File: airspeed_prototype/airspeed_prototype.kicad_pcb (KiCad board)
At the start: 2 copper layers, 2 parts, among them U1 BME280, U2 ADXL343

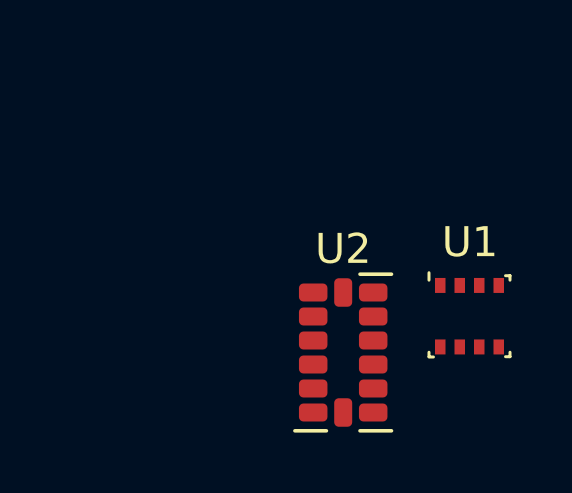
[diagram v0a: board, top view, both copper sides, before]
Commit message: test
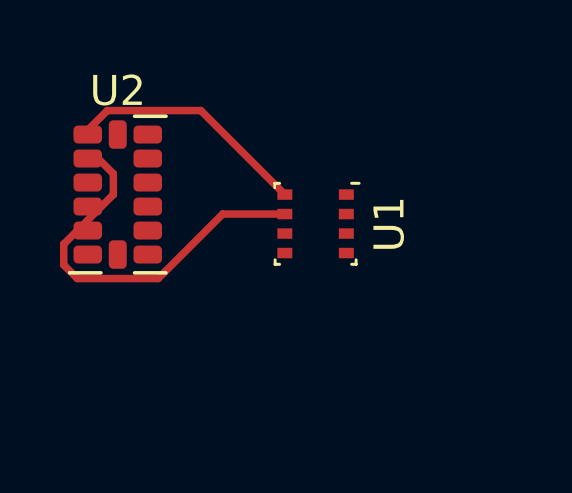
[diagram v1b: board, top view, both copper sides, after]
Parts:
- moved U2 9.18 mm to (134.6, 71.1)
- moved U1 5.98 mm to (141.2, 72.1), turned to -90 degrees
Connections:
- U1 pad 1: unconnected-(U1-GND-Pad1) -> GND
- U1 pad 7: unconnected-(U1-GND-Pad7) -> Net-(U1-GND-Pad7)
- U1 pad 8: unconnected-(U1-VDD-Pad8) -> +3.3V
- U2 pad 1: unconnected-(U2-Vdd_I/O-Pad1) -> +3.3V
- U2 pad 2: Net-(U2-GND-Pad2) -> Net-(U1-GND-Pad7)
- U2 pad 4: Net-(U2-GND-Pad2) -> Net-(U1-GND-Pad7)
- U2 pad 5: Net-(U2-GND-Pad2) -> Net-(U1-GND-Pad7)
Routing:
- net Net-(U1-GND-Pad7): track 0.00 -> 13.6 mm
- net +3.3V: track 0.00 -> 8.49 mm
